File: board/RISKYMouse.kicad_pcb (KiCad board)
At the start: 4 copper layers, 17.9 x 29.3 mm, 20 parts, among them J1 DE9_Plug, J2 Conn_01x02, J3 USB_1, U1 CH32V203C8T6, U2 LM1117MP-3.3

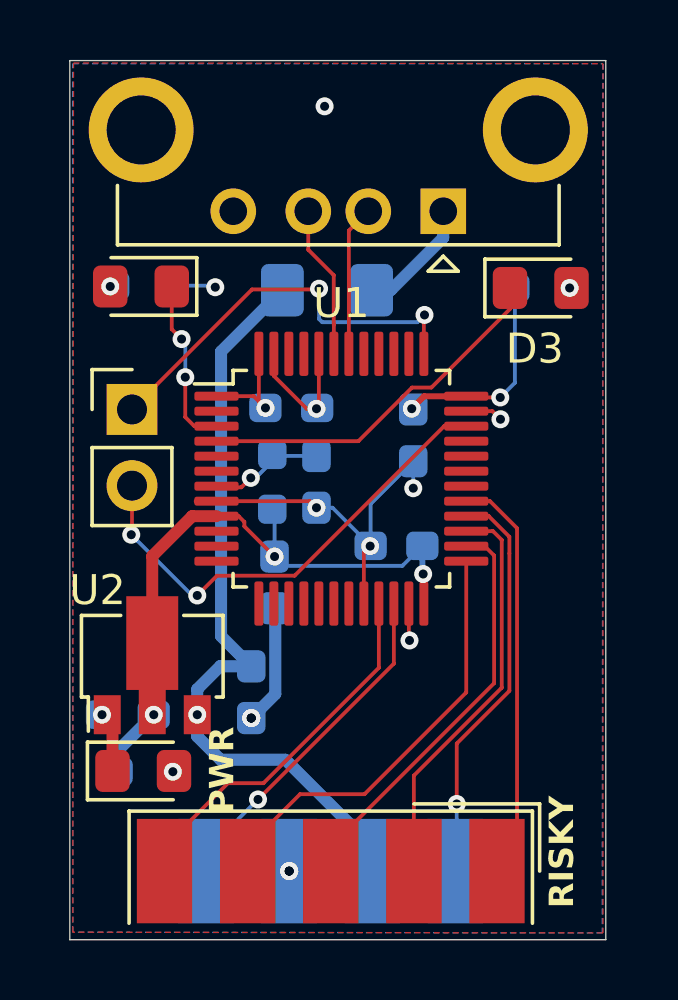
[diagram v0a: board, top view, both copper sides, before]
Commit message: revised PCB
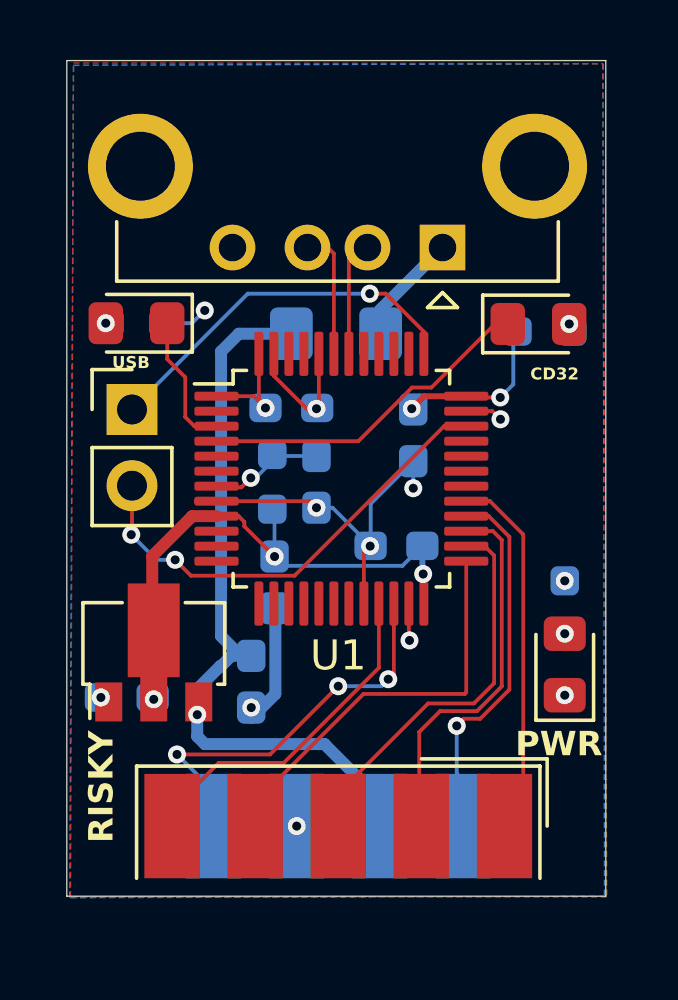
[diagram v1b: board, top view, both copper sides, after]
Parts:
- moved R1 15.0 mm to (137.7, 94.5), turned to 90 degrees
- moved D1 14.5 mm to (137.7, 96.4), turned to 90 degrees
- moved J1 1.52 mm to (130.2, 101.8)
- moved F1 1.48 mm to (130.1, 85.3)
- moved R4 1.45 mm to (137.1, 85.3)
- moved R3 1.26 mm to (123.5, 85.0)
- moved D2 1.23 mm to (123.5, 85.0)
- moved J3 1.21 mm to (133.7, 82.5)
- moved D3 1.20 mm to (136.8, 85.0)
- moved C1 0.58 mm to (123.1, 97.5)
- moved U2 0.43 mm to (124.0, 95.7)
- moved C4 0.35 mm to (127.3, 97.0)
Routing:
- net +3.3V: track 34.8 -> 30.6 mm, vias 7 -> 8
- net /PIN9: track 11.5 -> 14.4 mm, vias 1 -> 3
- net /PIN1: track 15.0 -> 12.2 mm
- net GND: track 25.7 -> 23.8 mm, vias 12 -> 10
- net /USB_DP: track 6.04 -> 4.44 mm
- net /PIN6: track 13.6 -> 12.3 mm
- net /SWCLK: track 13.9 -> 12.6 mm, vias 2 -> 1
- net /LED1: track 5.71 -> 4.54 mm, vias 2 -> 0
- net /PIN5: track 12.6 -> 11.4 mm
- net /PIN4: track 14.6 -> 13.6 mm
- net /PIN2: track 13.6 -> 12.5 mm
- net /LED2: track 12.3 -> 11.3 mm
- net +5V: track 25.7 -> 24.8 mm
- net /PIN3: track 13.8 -> 13.0 mm
- net /USB_DM: track 5.02 -> 4.42 mm
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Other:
- board size 17.9 x 29.3 mm -> 18 x 27.9 mm
- board text added: "CD32"
- board text added: "USB"
